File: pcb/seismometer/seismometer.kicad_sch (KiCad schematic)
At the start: 49 parts

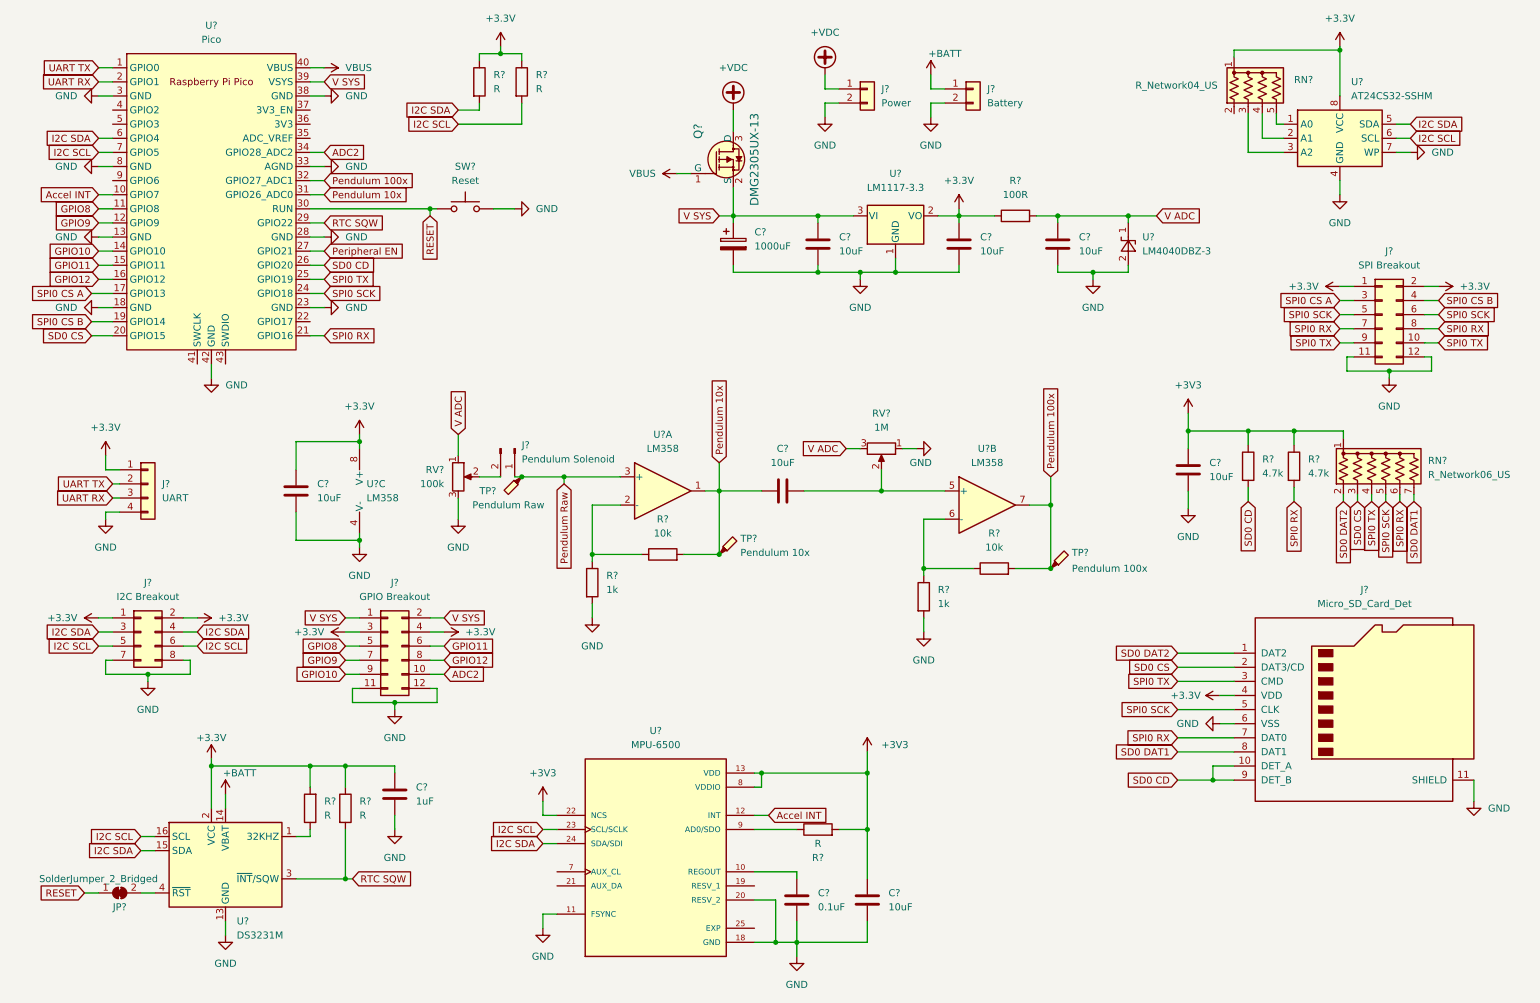
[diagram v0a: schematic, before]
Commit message: Updating PCB Schematic
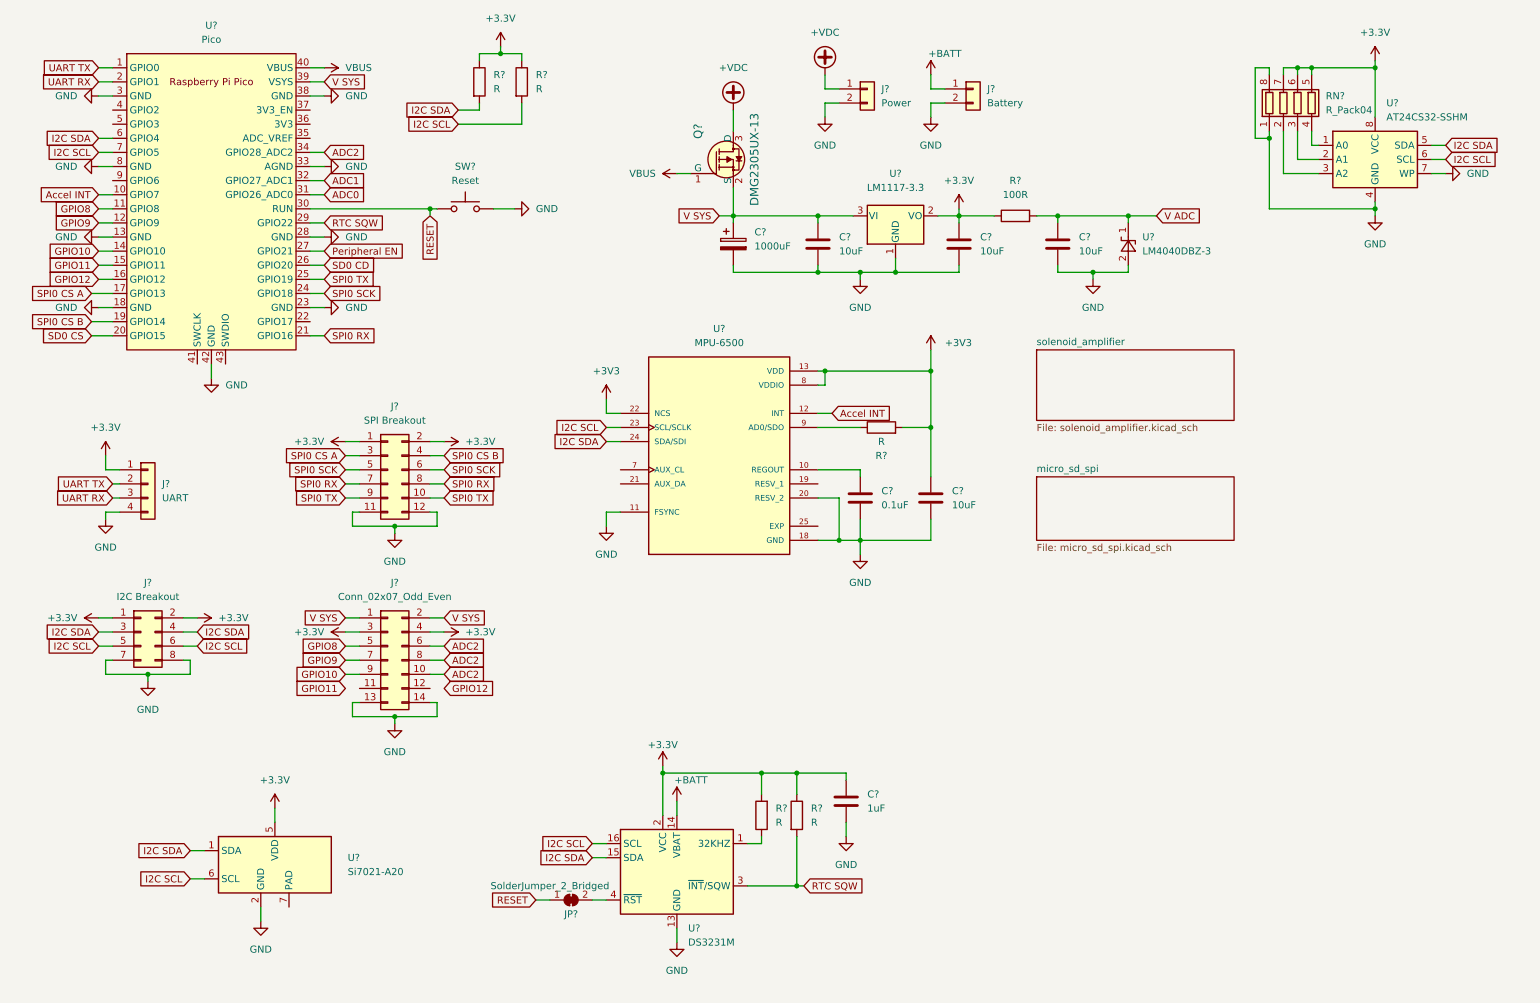
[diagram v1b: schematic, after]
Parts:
- removed C? (x3): 10uF, symbol Device:C
- removed J?: GPIO Breakout, symbol Connector_Generic:Conn_02x06_Odd_Even
- removed J?: Pendulum Solenoid, symbol Connector:Conn_01x02_Male
- removed J?: Micro_SD_Card_Det, symbol Connector:Micro_SD_Card_Det
- removed R? (x2): 1k, symbol Device:R
- removed R? (x2): 4.7k, symbol Device:R
- removed R? (x2): 10k, symbol Device:R
- removed RN?: R_Network04_US, Resistor_THT:R_Array_SIP5, symbol Device:R_Network04_US
- removed RN?: R_Network06_US, Resistor_THT:R_Array_SIP7, symbol Device:R_Network06_US
- removed RV?: 1M, symbol Device:R_Potentiometer
- removed RV?: 100k, symbol Device:R_Potentiometer
- removed TP?: Pendulum Raw, symbol Connector:TestPoint_Probe
- removed TP?: Pendulum 10x, symbol Connector:TestPoint_Probe
- removed TP?: Pendulum 100x, symbol Connector:TestPoint_Probe
- removed U? (x3): LM358, symbol Amplifier_Operational:LM358
- added J?: Conn_02x07_Odd_Even, symbol Connector_Generic:Conn_02x07_Odd_Even
- added RN?: R_Pack04, symbol Device:R_Pack04
- added U?: Si7021-A20, Package_DFN_QFN:DFN-6-1EP_3x3mm_P1mm_EP1.5x2.4mm, symbol Sensor_Humidity:Si7021-A20
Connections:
- net +3.3V: now also J?.3 (Pin_3), J?.4 (Pin_4), RN?.5 (R4.2), RN?.6 (R3.2), RN?.7 (R2.2), U?.5 (VDD)
- net ADC2: now also J?.10 (Pin_10), J?.6 (Pin_6), J?.8 (Pin_8)
- net GND: now also J?.13 (Pin_13), J?.14 (Pin_14), RN?.1 (R1.1), RN?.8 (R1.2), U?.2 (GND)
- net GPIO10: now also J?.9 (Pin_9)
- net GPIO8: now also J?.5 (Pin_5)
- net GPIO9: now also J?.7 (Pin_7)
- net I2C SCL: now also U?.6 (SCL)
- net I2C SDA: now also U?.1 (SDA)
- net V SYS: now also J?.1 (Pin_1), J?.2 (Pin_2)
- net at U?.3 (A2): now also RN?.2 (R2.1)
- net at U?.2 (A1): now also RN?.3 (R3.1)
- net at U?.1 (A0): now also RN?.4 (R4.1)
- net Pendulum 100x renamed ADC1
- net Pendulum 10x renamed ADC0
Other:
- added sheet micro_sd_spi (micro_sd_spi.kicad_sch)
- added sheet solenoid_amplifier (solenoid_amplifier.kicad_sch)
- moved on the sheet: C?, J?, JP?, R?, U?
